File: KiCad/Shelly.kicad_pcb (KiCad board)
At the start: 2 copper layers, 14 x 28 mm, 26 parts, among them J1 Shelly 1, J2 Other, J3 USB-C, Q1 PMF170XP,115, Q2 PMF250XNEX, U1 FT231XQ, U2 LMR16006+FB

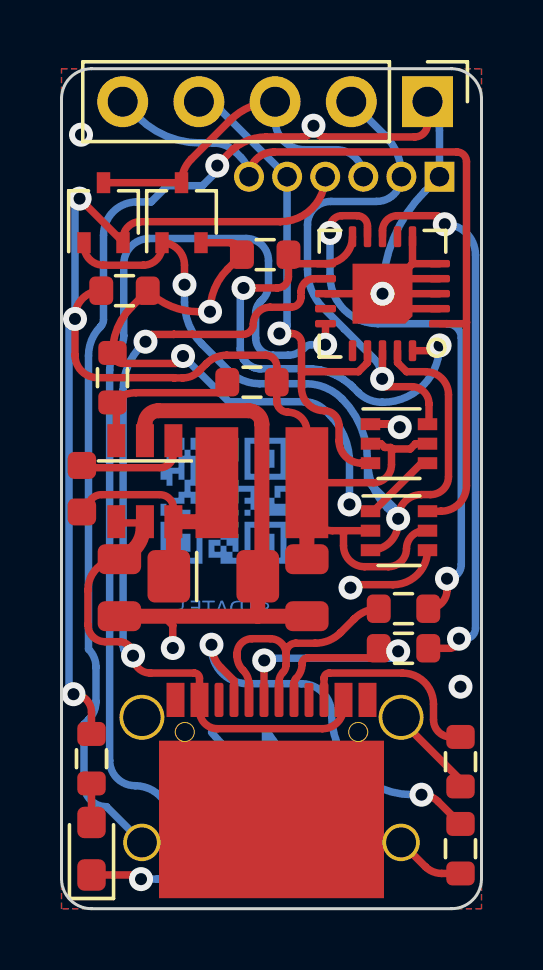
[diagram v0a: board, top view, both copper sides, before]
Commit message: Library update
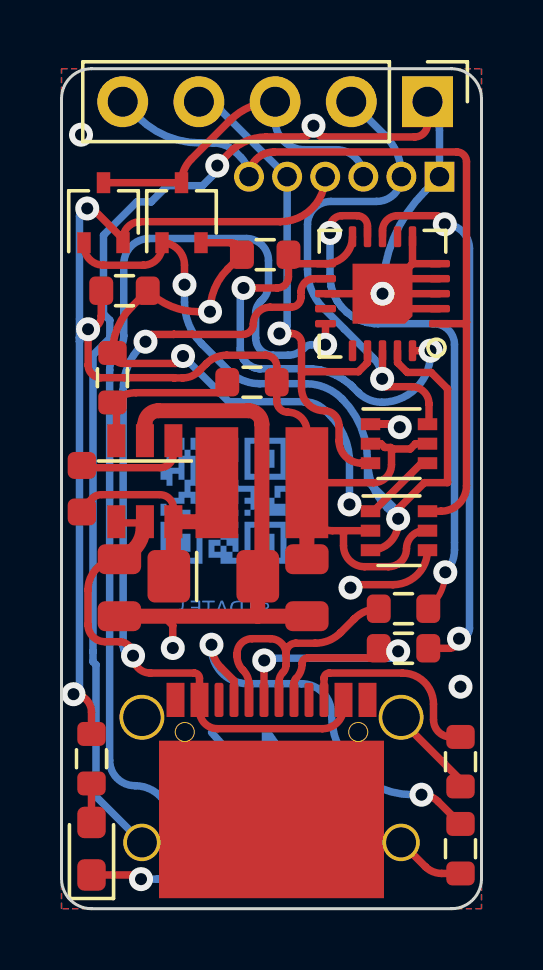
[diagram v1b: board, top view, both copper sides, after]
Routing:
- net Net-(C1-Pad1): track 16.6 -> 15.9 mm
- net +3V3: track 55.8 -> 55.1 mm
- net D-: track 18.7 -> 18.1 mm
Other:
- rule pad_to_mask_clearance: 0 -> 0.01

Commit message: PCB
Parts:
- added ?: , RevK:PasteTasmotizer, F.Cu at (164.1, 95.2)
